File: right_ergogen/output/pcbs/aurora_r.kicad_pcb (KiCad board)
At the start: 2 copper layers, 161.2 x 132.9 mm, 124 parts

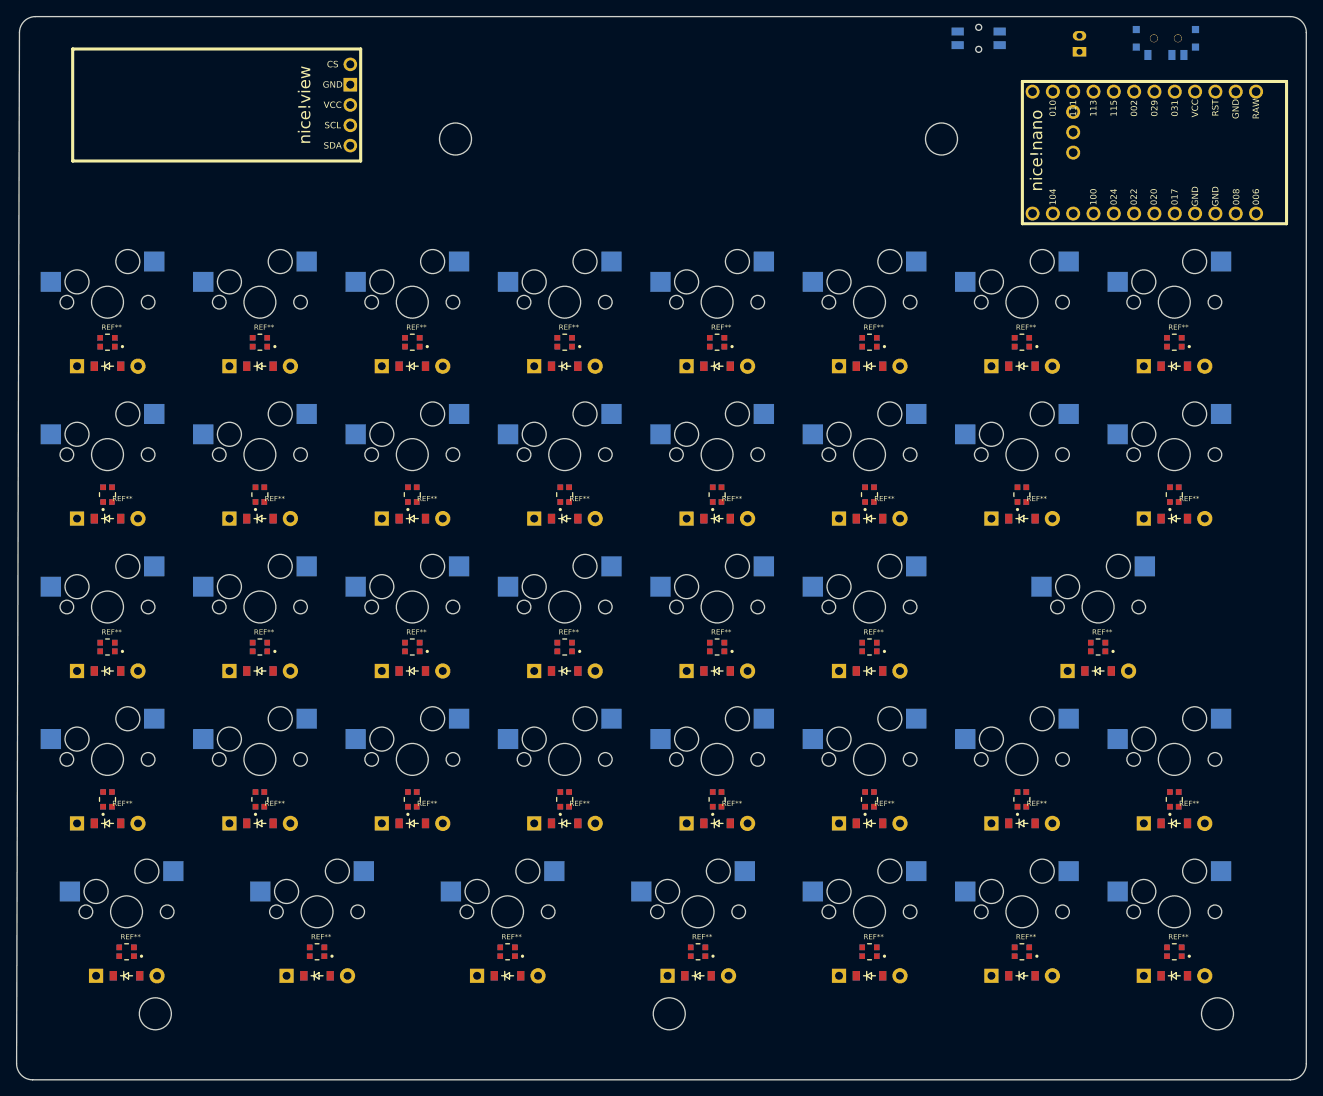
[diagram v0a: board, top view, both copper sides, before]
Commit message: Generate output CAD files
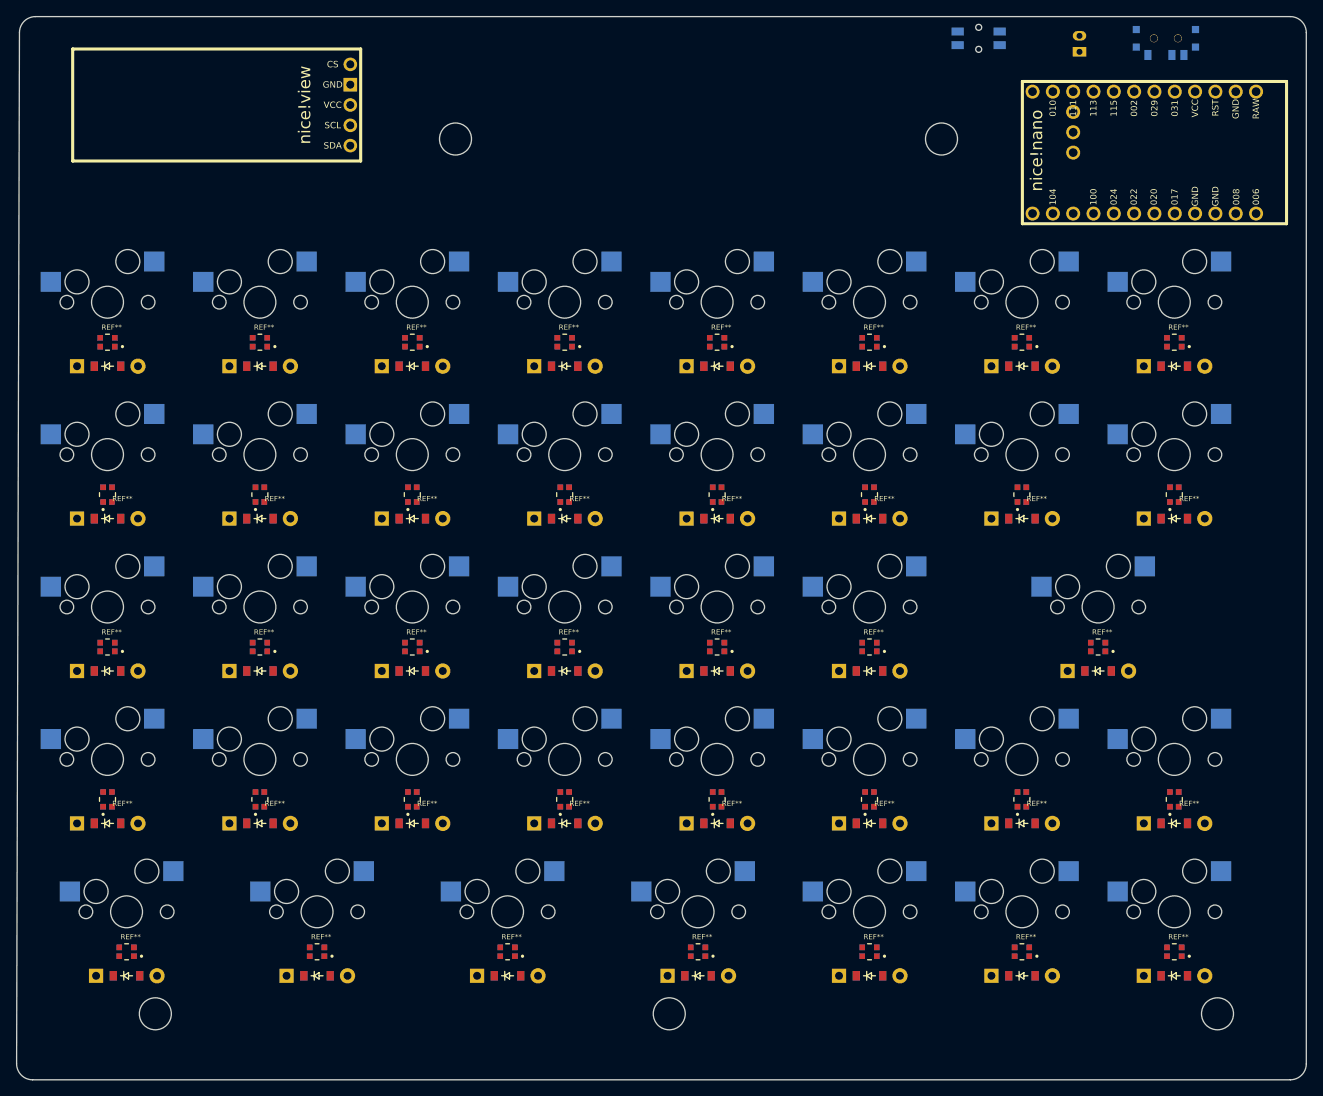
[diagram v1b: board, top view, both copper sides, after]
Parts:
- removed the ? at (143.5, 60.5)
- removed the ? at (106.0, 169.9)
- removed the ? at (204.2, 60.5)
- removed the ? at (238.8, 169.9)
- removed the REF** at (233.3, 162.2)
- removed the REF** at (223.8, 124.0)
- added ?: , HOLE_M2_TH, F.Cu at (143.5, 60.6)
- added ?: , HOLE_M2_TH, F.Cu at (204.2, 60.6)
- added ?: , HOLE_M2_TH, F.Cu at (106.0, 169.9)
- added ?: , HOLE_M2_TH, F.Cu at (238.8, 169.9)
- added REF**: WS2812, WS2812-2020, F.Cu at (223.8, 124.0)
- added REF**: WS2812, WS2812-2020, F.Cu at (233.4, 162.2)
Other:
- net class Default added: clearance 0.2, trace_width 0.25, via_dia 0.8, via_drill 0.4
